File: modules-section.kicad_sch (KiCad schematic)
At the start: 26 parts, among them U1 ESP32-C3-DevKitM-1, U10 ADXL343, U11 WIZFI360-PA, U12 L86

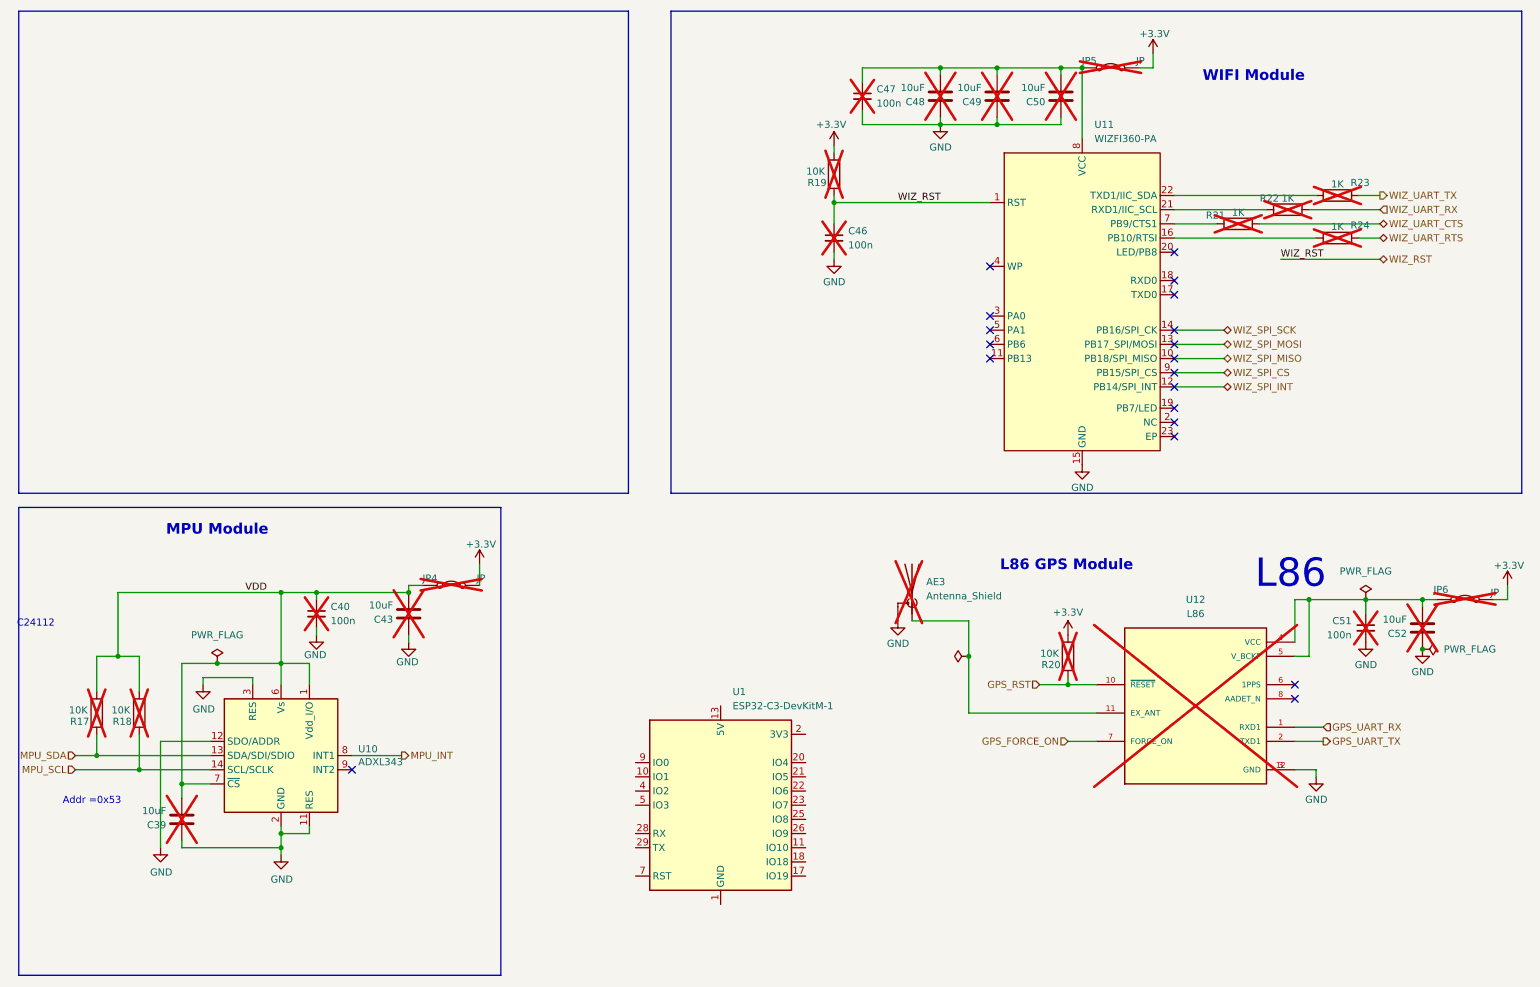
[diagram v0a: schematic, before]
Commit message: update the design
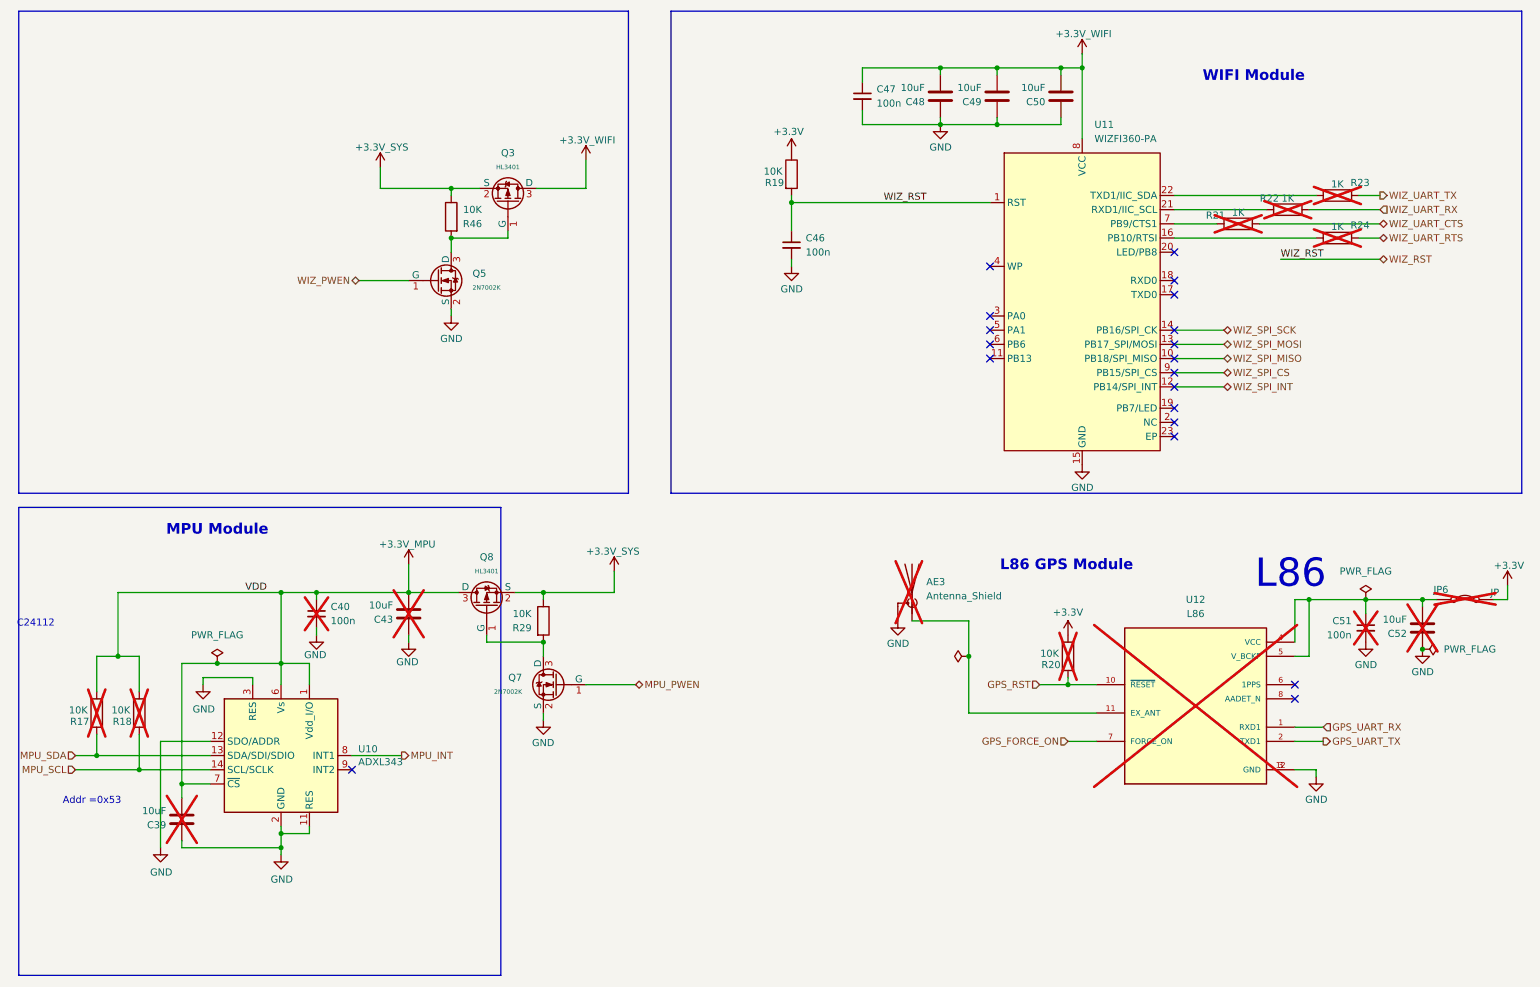
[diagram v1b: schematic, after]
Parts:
- removed JP4, JP5: JP, Jumper:SolderJumper-2_P1.3mm_Open_RoundedPad1.0x1.5mm, symbol Jumper:Jumper_2_Bridged
- removed U1: ESP32-C3-DevKitM-1, RF_Module:ESP32-C3-DevKitM-1, symbol RF_Module:ESP32-C3-DevKitM-1
- added Q3, Q8: HL3401, PCM_JLCPCB:Q_SOT-23, symbol PCM_JLCPCB-Transistors:PMOS,HL3401
- added Q5, Q7: 2N7002K, PCM_JLCPCB:Q_SOT-23, symbol PCM_JLCPCB-Transistors:NMOS,2N7002K
- added R29, R46: 10K, Resistor_SMD:R_0402_1005Metric, symbol Device:R
- C39: footprint Capacitor_SMD:C_0603_1608Metric -> Capacitor_SMD:C_0402_1005Metric
- C46, C47, C48, C49, C50, R19: now fitted
- R17, R18: footprint Resistor_SMD:R_0603_1608Metric -> Resistor_SMD:R_0402_1005Metric
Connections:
- net GND: now also Q5.2 (S), Q7.2 (S)
- net +3.3V_WIFI: now reaches C47.1, C48.1, C49.1, C50.1, U11.8 (VCC)
- net +3.3V_WIFI: now also Q3.3 (D)
- net VDD renamed +3.3V_MPU
- net +3.3V_MPU: now also Q8.3 (D)
- new net: Q7.3 (D), Q8.1 (G), R29.2
- new net: Q3.1 (G), Q5.3 (D), R46.2
- new net +3.3V_SYS: Q3.2 (S), Q8.2 (S), R29.1, R46.1
- new net MPU_PWEN: Q7.1 (G)
- new net WIZ_PWEN: Q5.1 (G)
